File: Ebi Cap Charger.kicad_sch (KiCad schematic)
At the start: 1 part

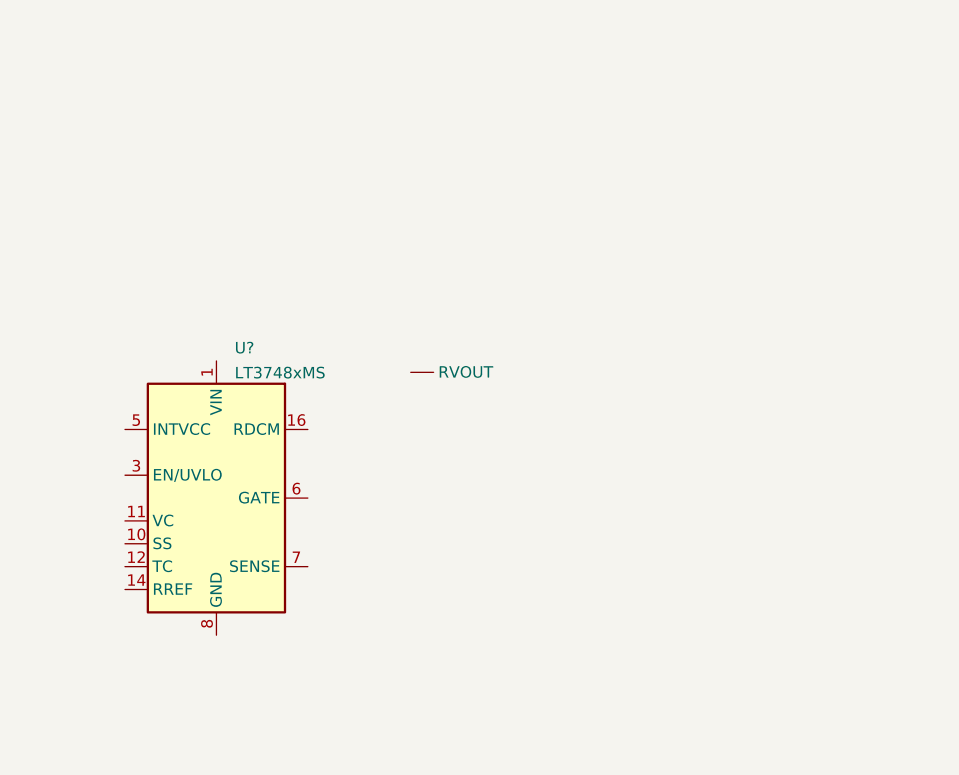
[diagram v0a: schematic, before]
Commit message: Started schematic
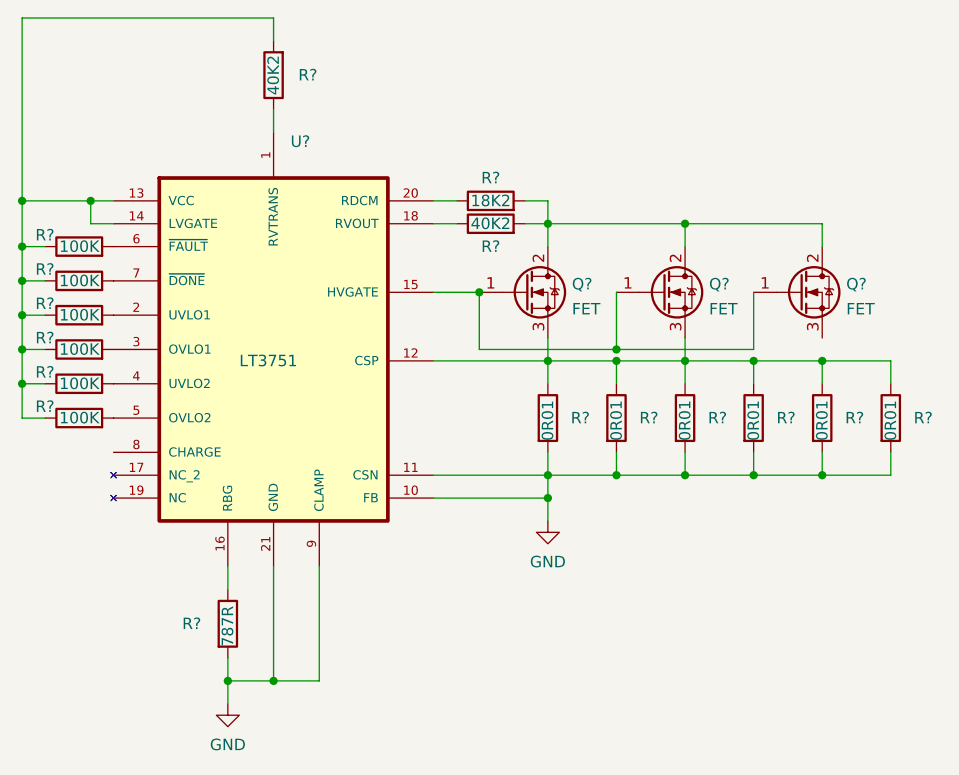
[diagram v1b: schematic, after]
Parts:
- removed U?: LT3748xMS, Package_SO:Linear_MSOP-12-16_3x4mm_P0.5mm, symbol Regulator_Switching:LT3748xMS
- added Q? (x3): FET, symbol Device:Q_NMOS_GDS
- added R? (x6): 0R01, symbol Device:R
- added R?: 787R, symbol Device:R
- added R? (x6): 100K, symbol Device:R
- added R?: 18K2, symbol Device:R
- added R? (x2): 40K2, symbol Device:R
- added U?: LT3751, SOP65P640X120-21N, symbol LT3751:LT3751IFEPBF
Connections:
- new net: Q?.3 (S), Q?.3 (S), R?.1, R?.1, R?.1, R?.1, R?.1, R?.1, U?.12 (CSP)
- new net: R?.1, U?.16 (RBG)
- new net: R?.1, R?.1, R?.1, R?.1, R?.1, R?.1, R?.2, U?.13 (VCC), U?.14 (LVGATE)
- new net: R?.2, U?.6 (~{FAULT})
- new net: Q?.1 (G), Q?.1 (G), Q?.1 (G), U?.15 (HVGATE)
- new net: Q?.2 (D), Q?.2 (D), Q?.2 (D), R?.2, R?.2
- new net: R?.2, U?.3 (OVLO1)
- new net: R?.2, U?.7 (~{DONE})
- new net: R?.1, U?.20 (RDCM)
- new net: R?.2, U?.2 (UVLO1)
- new net: R?.2, U?.4 (UVLO2)
- new net: R?.2, U?.5 (OVLO2)
- new net: R?.1, U?.1 (RVTRANS)
- new net: R?.1, U?.18 (RVOUT)
- new net GND: R?.2, R?.2, R?.2, R?.2, R?.2, R?.2, R?.2, U?.10 (FB), U?.11 (CSN), U?.21 (GND), U?.9 (CLAMP)
